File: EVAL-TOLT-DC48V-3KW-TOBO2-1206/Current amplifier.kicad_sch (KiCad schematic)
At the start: 27 parts, among them J1 V_BAT+, J2 V_BAT-

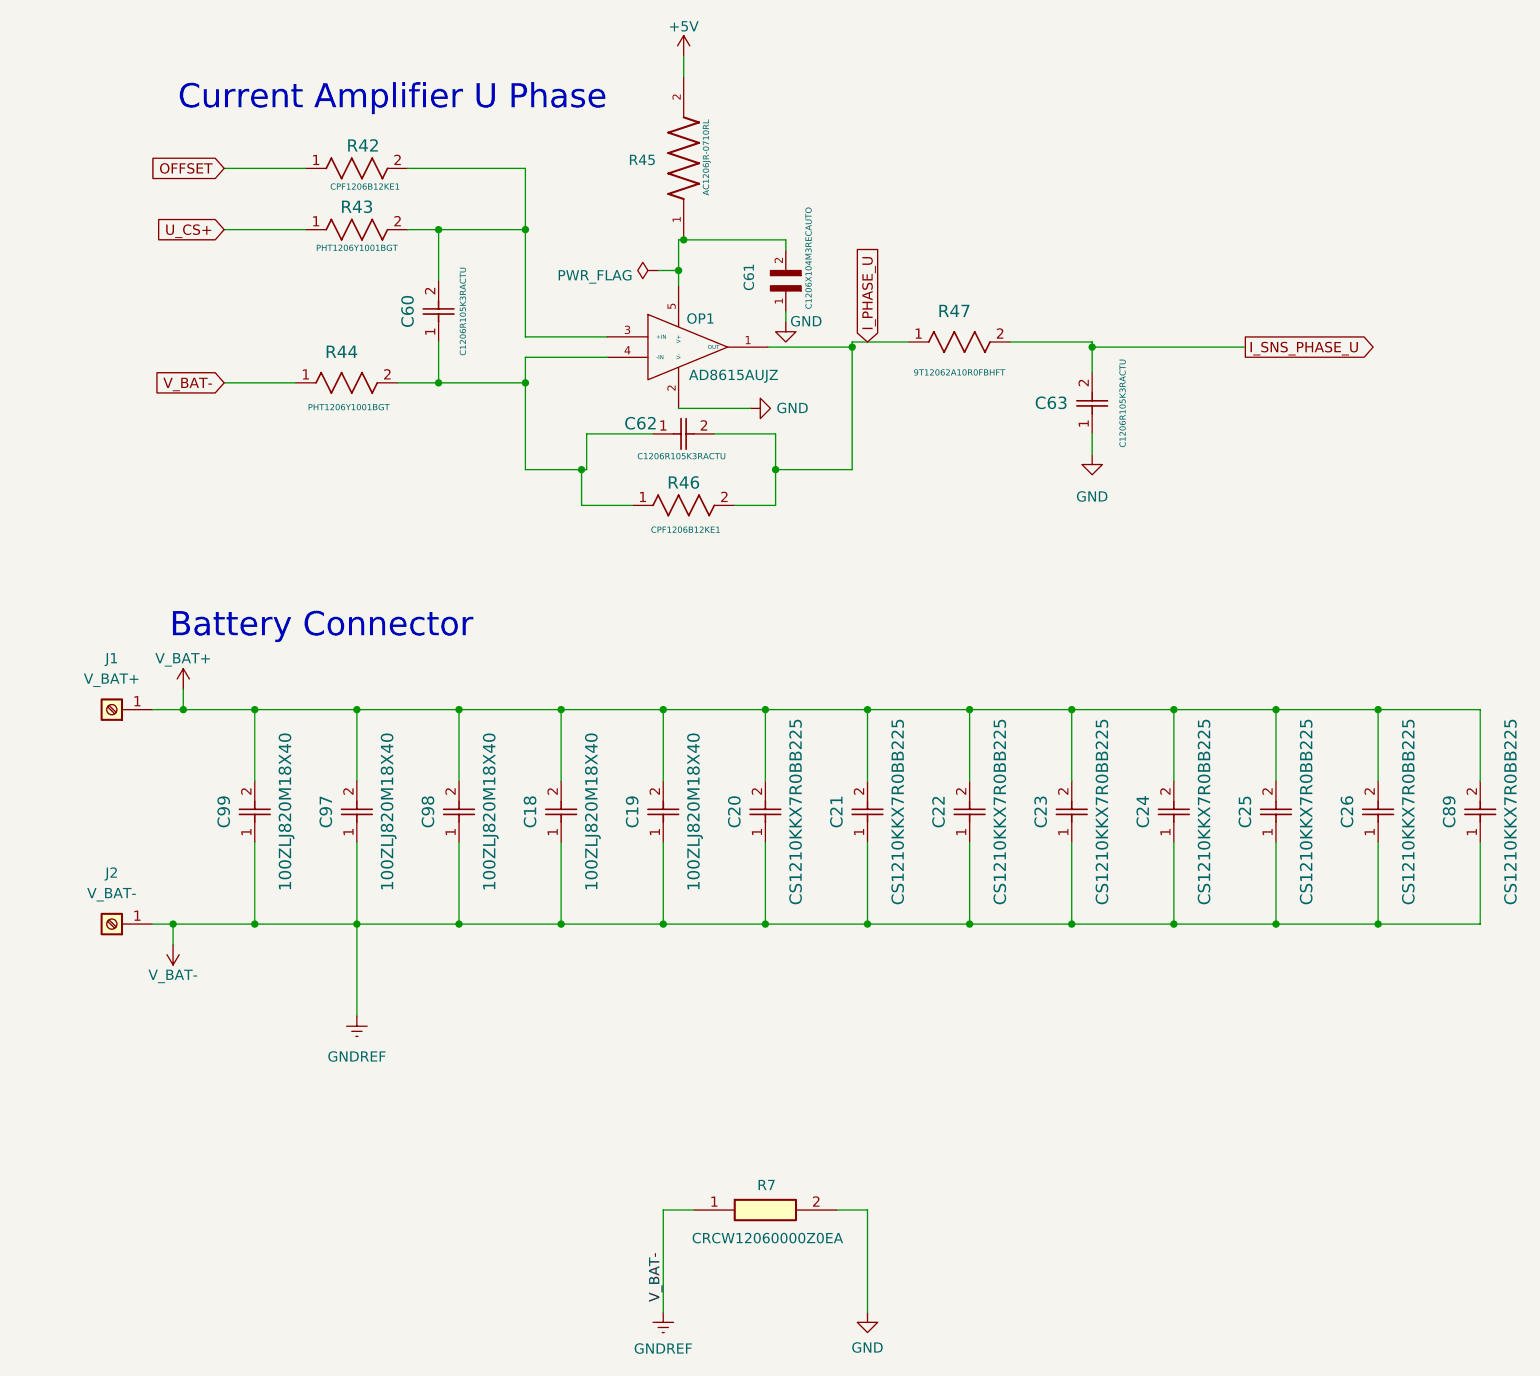
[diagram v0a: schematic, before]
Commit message: v10112024-2
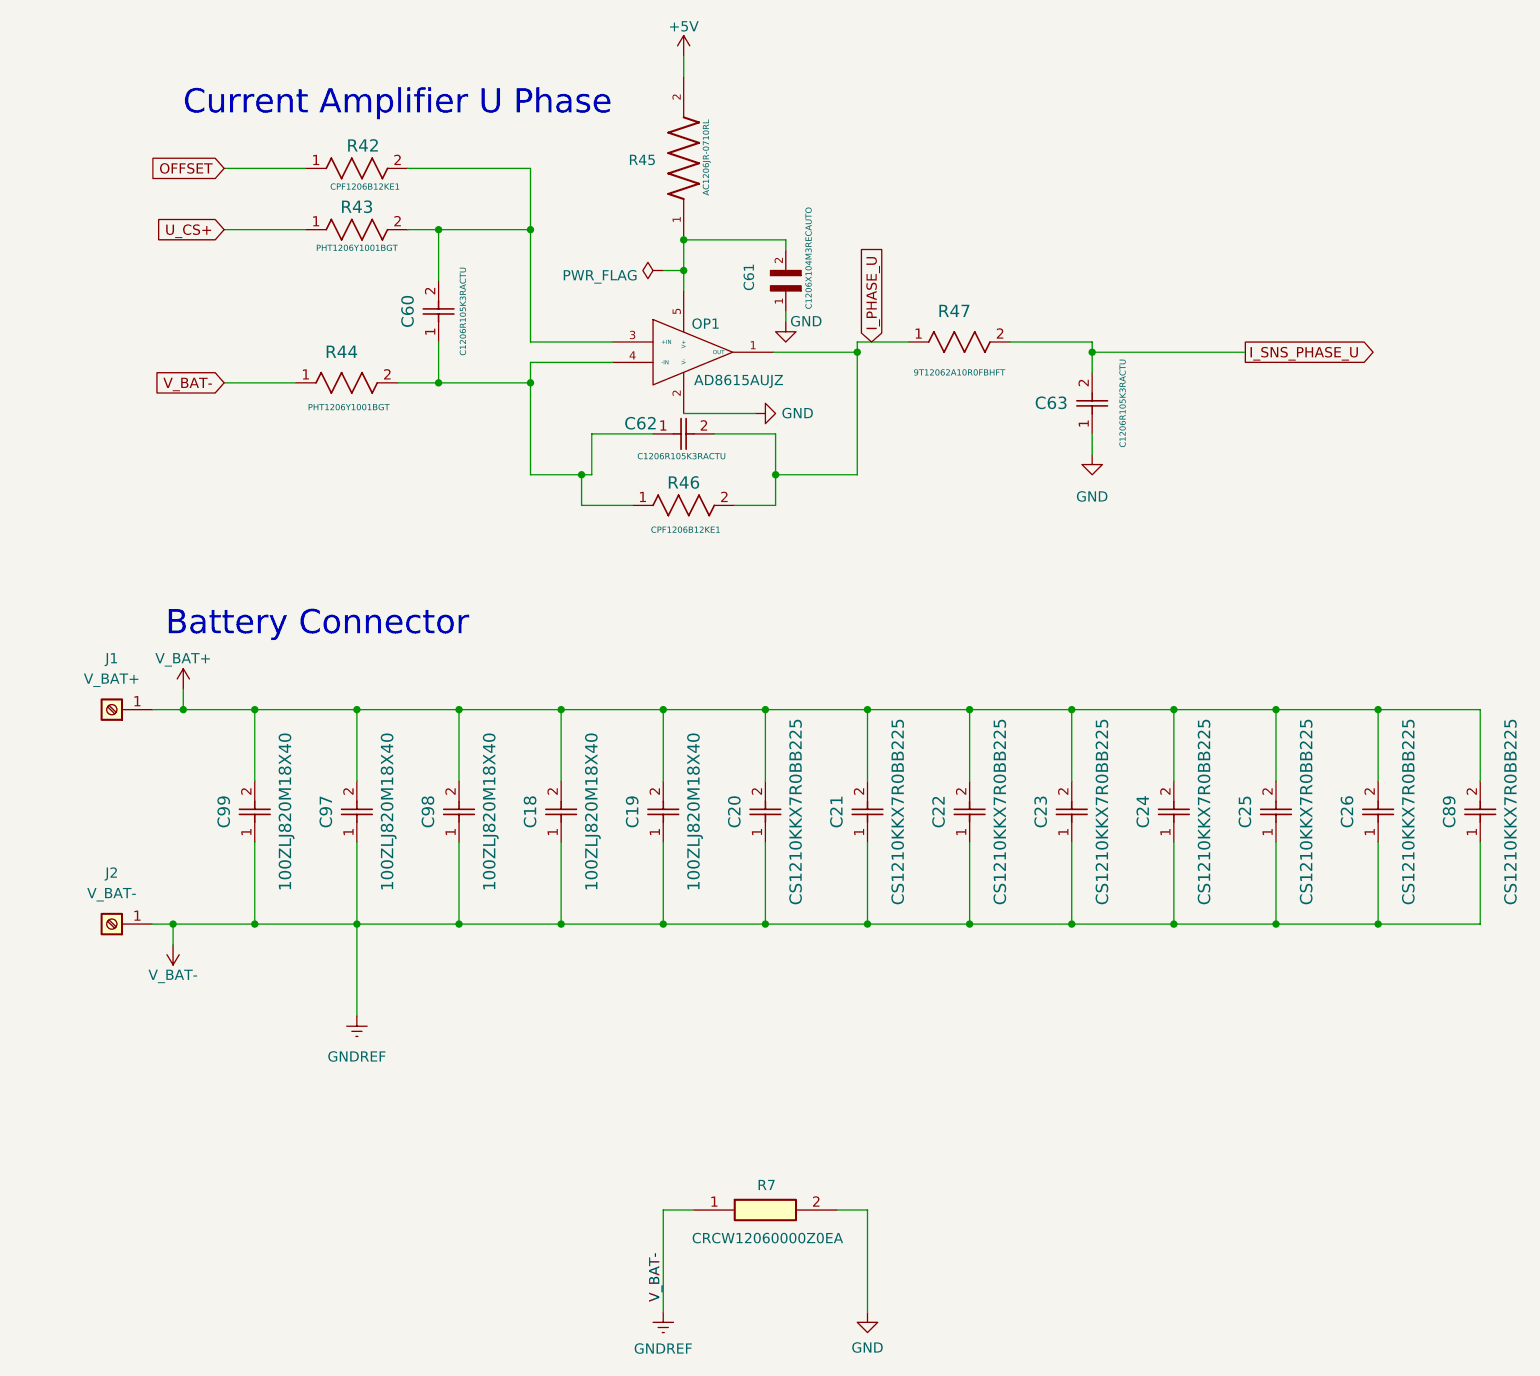
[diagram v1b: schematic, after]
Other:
- moved on the sheet: OP1
